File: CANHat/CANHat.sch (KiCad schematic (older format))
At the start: 1 part, among them J0 RPi_GPIO

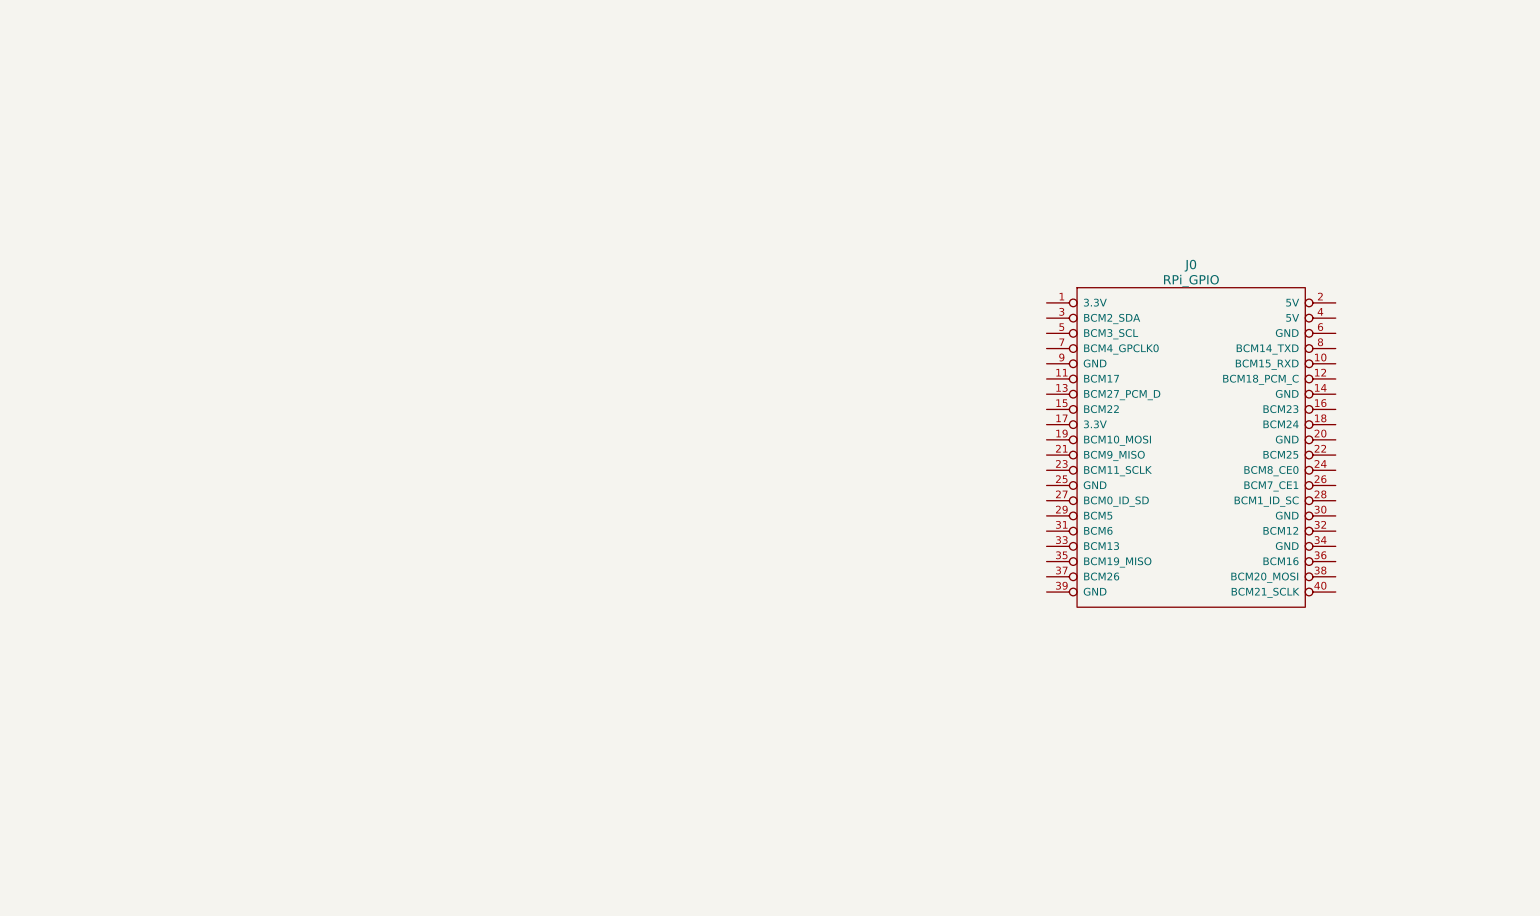
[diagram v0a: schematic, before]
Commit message: Small typo error fixed
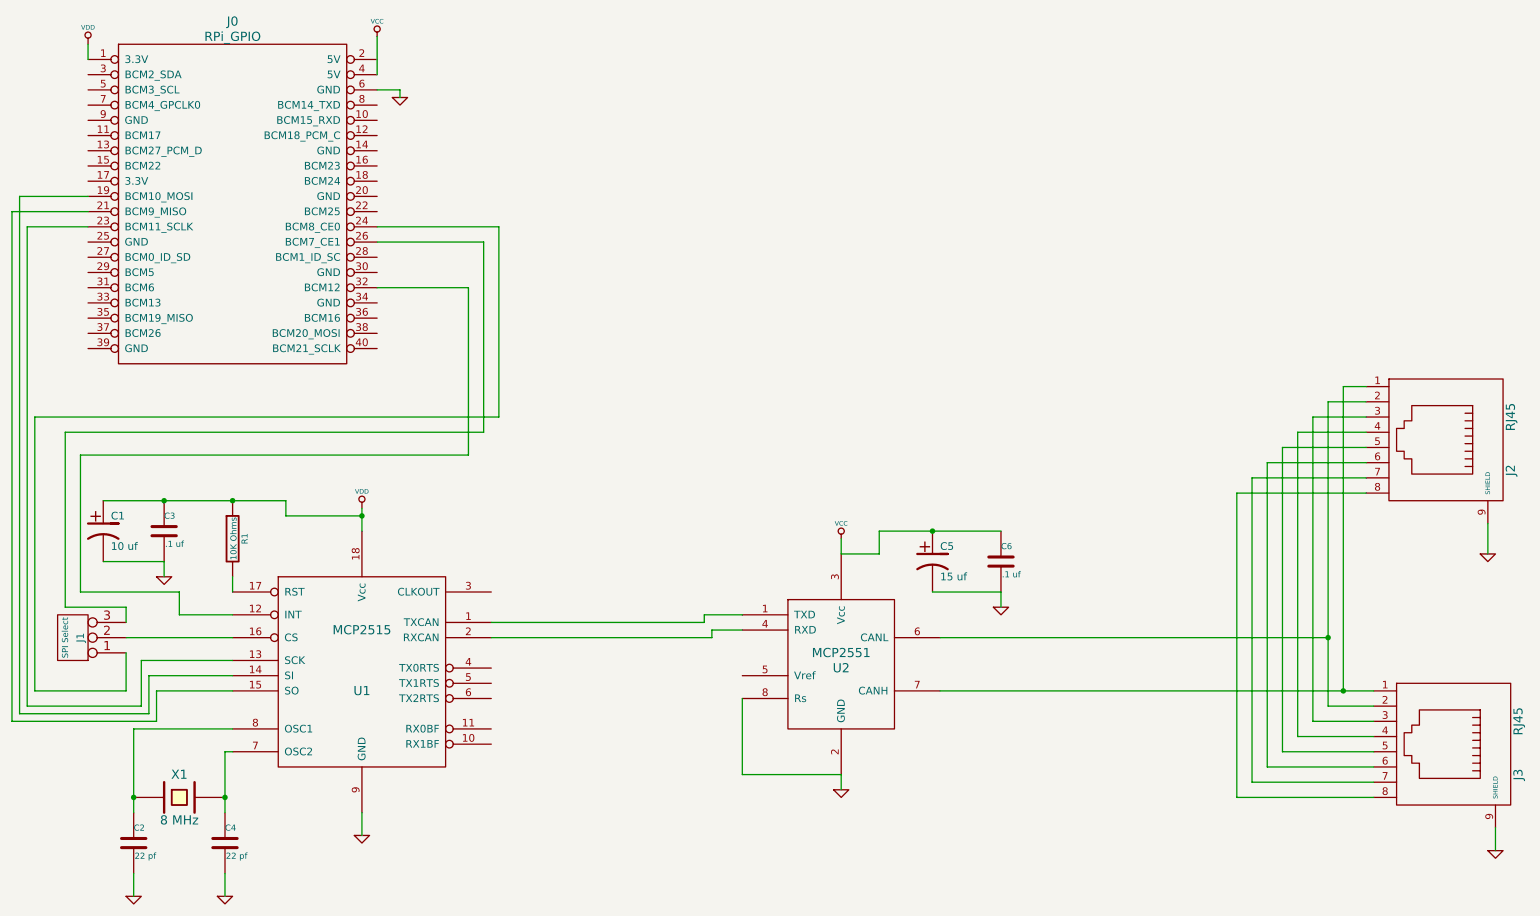
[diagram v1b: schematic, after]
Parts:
- added C1: 10 uf, ~, symbol CP1
- added C2, C4: 22 pf, ~, symbol C
- added C3, C6: .1 uf, ~, symbol C
- added C5: 15 uf, ~, symbol CP1
- added J1: SPI Select, SIL-3, symbol CONN_3
- added J2, J3: RJ45, ~, symbol RJ45
- added R1: 10K Ohms, ~, symbol R
- added U1: MCP2515, DIL-18_300, symbol MCP2515
- added U2: MCP2551, DIL-8_300, symbol MCP2551
- added X1: 8 MHz, ~, symbol CRYSTAL
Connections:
- net VDD: now reaches J0.1 (3.3V)
- net VDD: now also C1.1, C3.1, R1.1, U1.18 (Vcc)
- net at J0.19 (BCM10_MOSI): now also U1.14 (SI)
- net at J0.21 (BCM9_MISO): now also U1.15 (SO)
- net at J0.23 (BCM11_SCLK): now also U1.13 (SCK)
- net at J0.24 (BCM8_CE0): now also J1.1 (P1)
- net at J0.26 (BCM7_CE1): now also J1.3 (P3)
- net at J0.32 (BCM12): now also U1.12 (INT)
- net VCC: now reaches J0.4 (5V)
- net VCC: now also C5.1, C6.1, U2.3 (Vcc)
- net GND: now reaches J0.6 (GND)
- net GND: now also C1.2, C2.2, C3.2, C4.2, C5.2, C6.2, J2.9 (SHIELD), J3.9 (SHIELD), U1.9 (GND), U2.2 (GND), U2.8 (Rs)
- new net: U1.1 (TXCAN), U2.1 (TXD)
- new net: J1.2 (PM), U1.16 (CS)
- new net: R1.2, U1.17 (RST)
- new net: U1.2 (RXCAN), U2.4 (RXD)
- new net: C4.1, U1.7 (OSC2), X1.2
- new net: C2.1, U1.8 (OSC1), X1.1
- new net: J2.2, J3.2, U2.6 (CANL)
- new net: J2.1, J3.1, U2.7 (CANH)
- new net: J2.3, J3.3
- new net: J2.4, J3.4
- new net: J2.5, J3.5
- new net: J2.6, J3.6
- new net: J2.7, J3.7
- new net: J2.8, J3.8
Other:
- moved on the sheet: J0
